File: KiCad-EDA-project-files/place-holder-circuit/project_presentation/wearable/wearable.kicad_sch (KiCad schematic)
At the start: 1 part, among them U1 ATMEGA328-PU

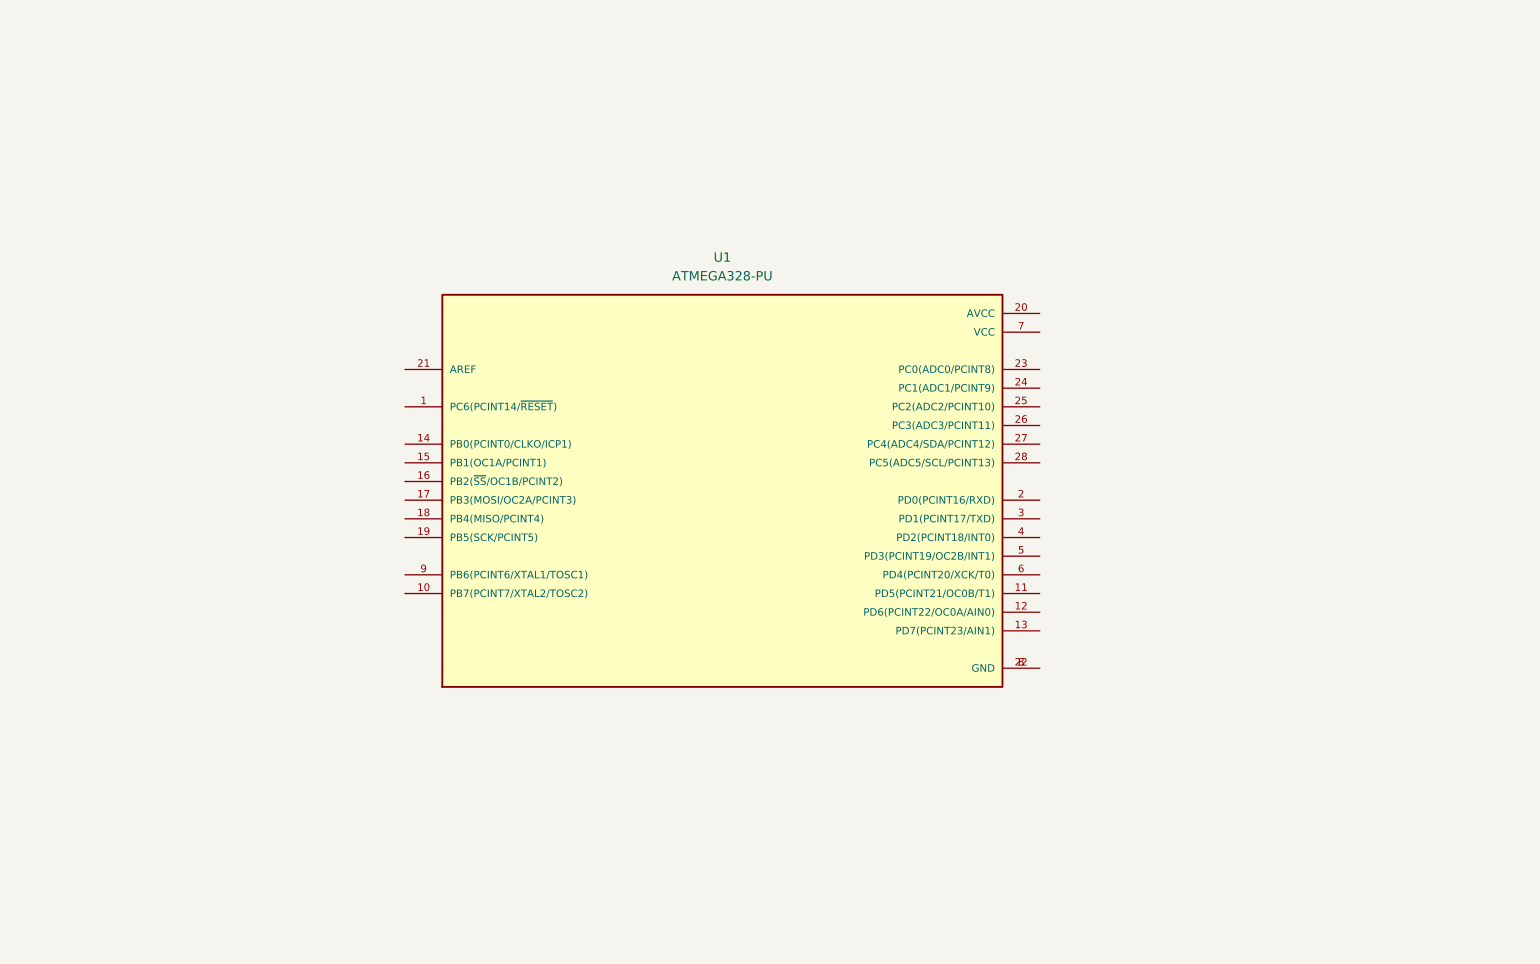
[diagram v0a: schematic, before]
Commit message: Arduino GPS code
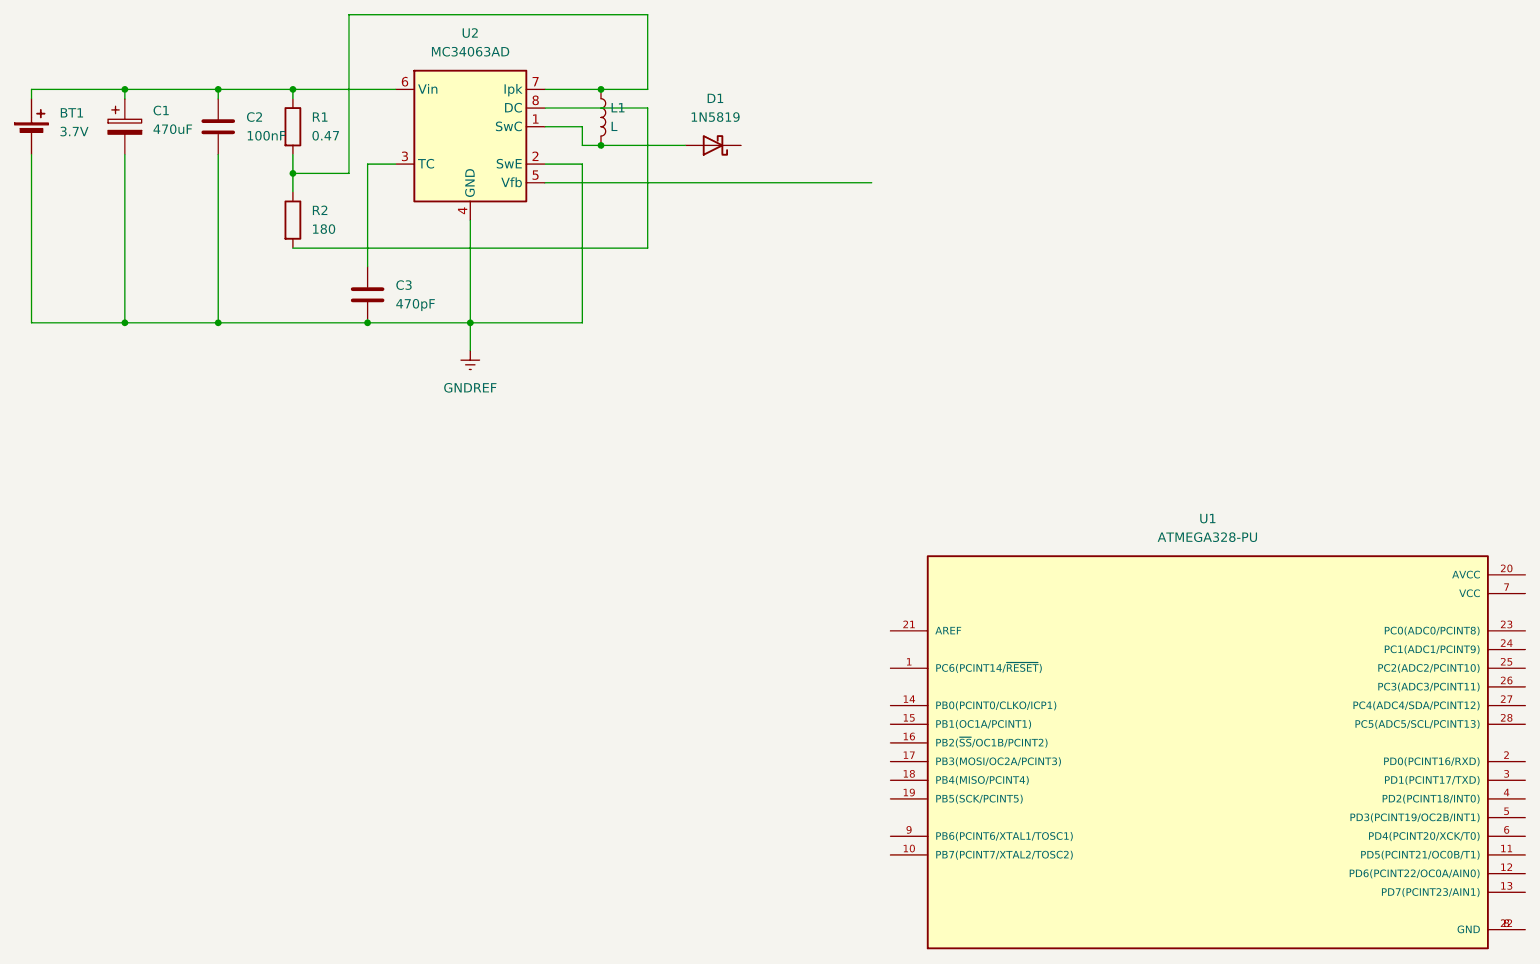
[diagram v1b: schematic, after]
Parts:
- added BT1: 3.7V, symbol Device:Battery_Cell
- added C1: 470uF, symbol Device:C_Polarized
- added C2: 100nF, symbol Device:C
- added C3: 470pF, symbol Device:C
- added D1: 1N5819, Diode_THT:D_DO-41_SOD81_P10.16mm_Horizontal, symbol Diode:1N5819
- added L1: L, symbol Device:L
- added R1: 0.47, symbol Device:R
- added R2: 180, symbol Device:R
- added U2: MC34063AD, Package_SO:SOIC-8_3.9x4.9mm_P1.27mm, symbol Regulator_Switching:MC34063AD
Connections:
- new net: D1.2 (A), L1.2, U2.1 (SwC)
- new net: BT1.1 (+), C1.1, C2.1, R1.1, U2.6 (Vin)
- new net: L1.1, R1.2, R2.1, U2.7 (Ipk)
- new net: R2.2, U2.8 (DC)
- new net: C3.1, U2.3 (TC)
- new net GNDREF: BT1.2 (-), C1.2, C2.2, C3.2, U2.2 (SwE), U2.4 (GND)
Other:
- moved on the sheet: U1
